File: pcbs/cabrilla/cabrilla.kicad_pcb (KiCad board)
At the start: 2 copper layers, 150 x 78 mm, 62 parts, among them J1 leds_velocidad, J10 Conn_01x10, J11 Conn_analogo, J12 inputs, J2 hm_1, J3 hm_2, J4 hm_3, J5 hm_4, J6 Conn_analogo, J7 Conn_01x08, J8 Conn_01x06, J9 Conn_01x08, K1 G5V-1, K2 G5V-1, Q1 Q_NPN_BEC, Q2 Q_NPN_BEC, SW1 SW_Push, SW2 SW_Push, U1 AZ1117-3.3, U2 STM32, U3 lorabee, Y1 lcd, Y2 LoRa

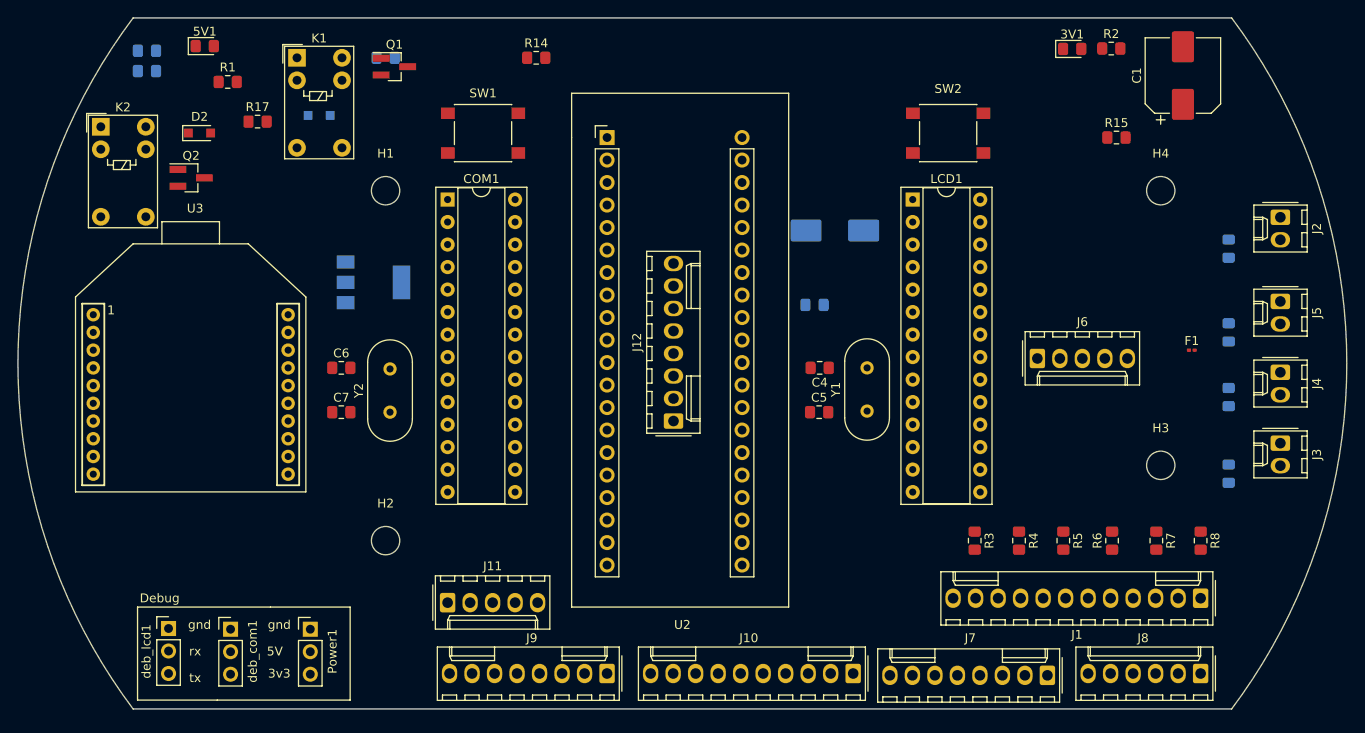
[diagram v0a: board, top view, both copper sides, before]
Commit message: Routed
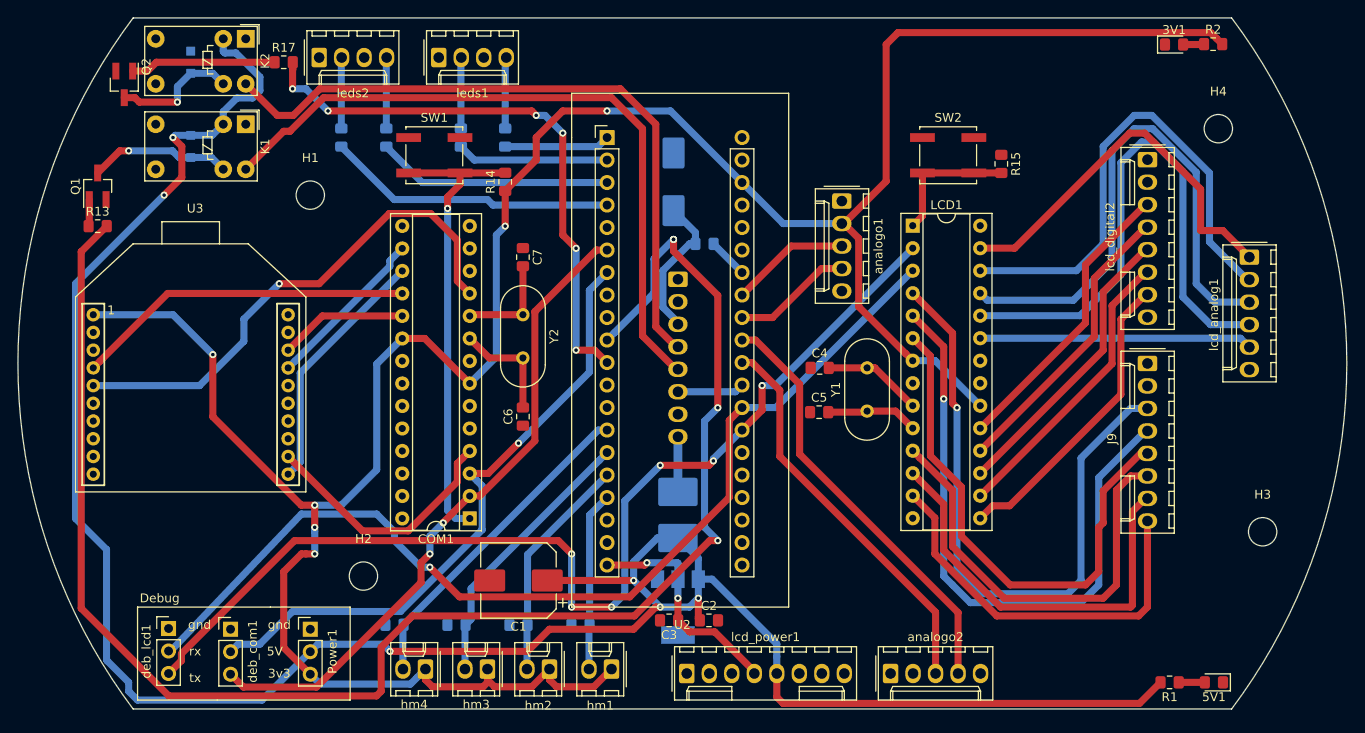
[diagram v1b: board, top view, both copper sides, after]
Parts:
- removed J1: leds_velocidad, Connector_Molex:Molex_KK-254_AE-6410-12A_1x12_P2.54mm_Vertical
- removed J10: Conn_01x10, Connector_Molex:Molex_KK-254_AE-6410-10A_1x10_P2.54mm_Vertical
- removed R5, R6: 10k, Resistor_SMD:R_0805_2012Metric_Pad1.15x1.40mm_HandSolder
- added lcd_power1: lcd_power, Connector_Molex:Molex_KK-254_AE-6410-08A_1x08_P2.54mm_Vertical, F.Cu at (139.5, 114.0)
- added leds1: Conn_01x04, Connector_Molex:Molex_KK-254_AE-6410-04A_1x04_P2.54mm_Vertical, F.Cu at (111.5, 44.5)
- added leds2: Conn_01x04, Connector_Molex:Molex_KK-254_AE-6410-04A_1x04_P2.54mm_Vertical, F.Cu at (98.0, 44.5)
- C2, C3, R13: moved to F.Cu
- D2, J12, R3, R4, R7, R8: moved to B.Cu
- F1: footprint Fuse:Fuse_0201_0603Metric -> Fuse:Fuse_2816_7142Metric_Pad3.20x4.45mm_HandSolder; moved to B.Cu
- J9: value Conn_01x08 -> lcd_digital1
- SW1, SW2: footprint Button_Switch_SMD:SW_Push_1P1T_NO_6x6mm_H9.5mm -> Button_Switch_SMD:SW_Push_1P1T_NO_CK_KSC6xxJ
- moved 5V1 134.7 mm to (199.0, 115.0), turned to 180 degrees
- moved R1 126.1 mm to (194.0, 115.0), turned to 180 degrees
- moved R8 107.1 mm to (100.5, 53.5), turned to 90 degrees
- moved hm4 105.0 mm to (110.0, 113.5), turned to 180 degrees
- moved R12 99.8 mm to (106.5, 108.5), turned to 0 degrees
- moved R7 98.1 mm to (105.6, 53.5), turned to 90 degrees
- moved hm3 95.6 mm to (117.0, 113.5), turned to 180 degrees
- moved C1 94.2 mm to (120.5, 103.5), turned to 180 degrees
- moved hm1 91.1 mm to (131.0, 113.5), turned to 180 degrees
- moved R11 90.9 mm to (113.5, 108.5), turned to 0 degrees
- moved C2 90.3 mm to (142.0, 108.0), turned to 0 degrees
- moved hm2 86.4 mm to (124.0, 113.5), turned to 180 degrees
- moved C3 85.5 mm to (137.5, 108.0)
- moved R9 84.6 mm to (127.5, 108.5), turned to 0 degrees
- moved R10 82.0 mm to (120.5, 108.5), turned to 0 degrees
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- renumbered J11 to analogo1, J6 to analogo2, J2 to hm1, J3 to hm2, J4 to hm3, J5 to hm4, J8 to lcd_analog1, J7 to lcd_digital2
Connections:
- net Net-(R16-Pad2) renamed /raw_pwm
- COM1 pad 11: Net-(COM1-Pad11) -> /Comunicaciones/RESET
- COM1 pad 4: Net-(COM1-Pad4) -> /Comunicaciones/DIO0
- F1 pad 2: +5V -> VCC
- J12 pad 2: +5V -> Net-(J12-Pad2)
- J12 pad 3: /corriente -> /pwm_motor
- J12 pad 4: /pwm_motor -> /freno
- J12 pad 6: /freno -> /corriente
- J12 pad 8: Net-(J12-Pad8) -> VCC
- J9 pad 3: Net-(J9-Pad3) -> /LCD/D2
- J9 pad 4: Net-(J9-Pad4) -> /LCD/D3
- J9 pad 5: Net-(J9-Pad5) -> /LCD/D4
- J9 pad 6: Net-(J9-Pad6) -> /LCD/D5
- J9 pad 7: Net-(J9-Pad7) -> /LCD/D6
- J9 pad 8: Net-(J9-Pad8) -> /LCD/D7
- LCD1 pad 11: Net-(LCD1-Pad11) -> /LCD/D5
- LCD1 pad 12: Net-(LCD1-Pad12) -> /LCD/D6
- LCD1 pad 13: Net-(LCD1-Pad13) -> /LCD/D7
- LCD1 pad 14: Net-(LCD1-Pad14) -> /LCD/D0
- LCD1 pad 15: Net-(LCD1-Pad15) -> /LCD/D1
- LCD1 pad 16: Net-(LCD1-Pad16) -> /LCD/SS
- LCD1 pad 17: Net-(LCD1-Pad17) -> /LCD/DI
- LCD1 pad 18: Net-(LCD1-Pad18) -> /LCD/DO
- LCD1 pad 19: Net-(LCD1-Pad19) -> /LCD/SCK
- LCD1 pad 22: Net-(LCD1-Pad22) -> GND
- LCD1 pad 4: Net-(LCD1-Pad4) -> /LCD/D2
- LCD1 pad 5: Net-(LCD1-Pad5) -> /LCD/D3
- LCD1 pad 6: Net-(LCD1-Pad6) -> /LCD/D4
- LCD1 pad 8: Net-(LCD1-Pad22) -> GND
- R7 pad 1: /led_m5 -> /led_m3
- R8 pad 1: /led_m6 -> /led_m4
- U2 pad 10: /hm_2 -> /reversa_signal
- U2 pad 11: /hm_1 -> /freno_signal
- U2 pad 13: /reversa_signal -> Net-(U2-Pad13)
- U2 pad 14: /freno_signal -> /hm_4
- U2 pad 15: /led_m5 -> /hm_3
- U2 pad 16: /led_m6 -> /hm_2
- U2 pad 17: Net-(U2-Pad17) -> /hm_1
- U2 pad 8: /hm_4 -> Net-(U2-Pad8)
- U2 pad 9: /hm_3 -> Net-(U2-Pad9)
- U3 pad 12: Net-(U3-Pad12) -> /Comunicaciones/DIO0
- U3 pad 5: Net-(U3-Pad5) -> /Comunicaciones/RESET
- analogo1 pad 3: /analog_x -> /analog_y
- analogo1 pad 4: /analog_y -> /analog_x
- lcd_analog1 pad 1: /LCD/RD -> /LCD/RST
- lcd_analog1 pad 2: /LCD/WR -> /LCD/CS
- lcd_analog1 pad 4: /LCD/CS -> /LCD/WR
- lcd_analog1 pad 5: /LCD/RST -> /LCD/RD
- lcd_digital2 pad 3: Net-(J7-Pad3) -> /LCD/SCK
- lcd_digital2 pad 4: Net-(J7-Pad4) -> /LCD/DO
- lcd_digital2 pad 5: Net-(J7-Pad5) -> /LCD/DI
- lcd_digital2 pad 6: Net-(J7-Pad6) -> /LCD/SS
- lcd_digital2 pad 7: Net-(J7-Pad7) -> /LCD/D1
- lcd_digital2 pad 8: Net-(J7-Pad8) -> /LCD/D0
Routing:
- net +3V3: track 0.00 -> 325.7 mm, vias 0 -> 8
- net +5V: track 0.00 -> 256.7 mm, vias 0 -> 6
- net /reversa_signal: track 0.00 -> 182.3 mm, vias 0 -> 4
- net /LCD/rx_lcd: track 0.00 -> 122.0 mm, vias 0 -> 6
- net /LCD/tx_lcd: track 0.00 -> 115.4 mm, vias 0 -> 1
- net /reversa: track 0.00 -> 78.5 mm
- net /freno: track 0.00 -> 77.0 mm
- net /Comunicaciones/rx_lora: track 0.00 -> 74.6 mm, vias 0 -> 2
- net /LCD/D2: track 0.00 -> 72.8 mm, vias 0 -> 1
- net /Comunicaciones/tx_lora: track 0.00 -> 71.4 mm, vias 0 -> 1
- net /LCD/D3: track 0.00 -> 70.2 mm, vias 0 -> 1
- net /freno_signal: track 0.00 -> 64.8 mm, vias 0 -> 6
- net /LCD/WR: track 0.00 -> 62.8 mm
- net /LCD/RS: track 0.00 -> 61.5 mm
- net /LCD/D4: track 0.00 -> 59.1 mm
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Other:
- net class Default: trace_width 0.25 -> 0.8
- net class entrada added: clearance 0.2, trace_width 1, via_dia 0.8, via_drill 0.4
